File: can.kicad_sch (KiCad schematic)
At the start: 14 parts, among them J1 RJ45_LED_Shielded, J2 RJ45_LED_Shielded, J3 Conn_01x04, SW1 SW_DIP_x02

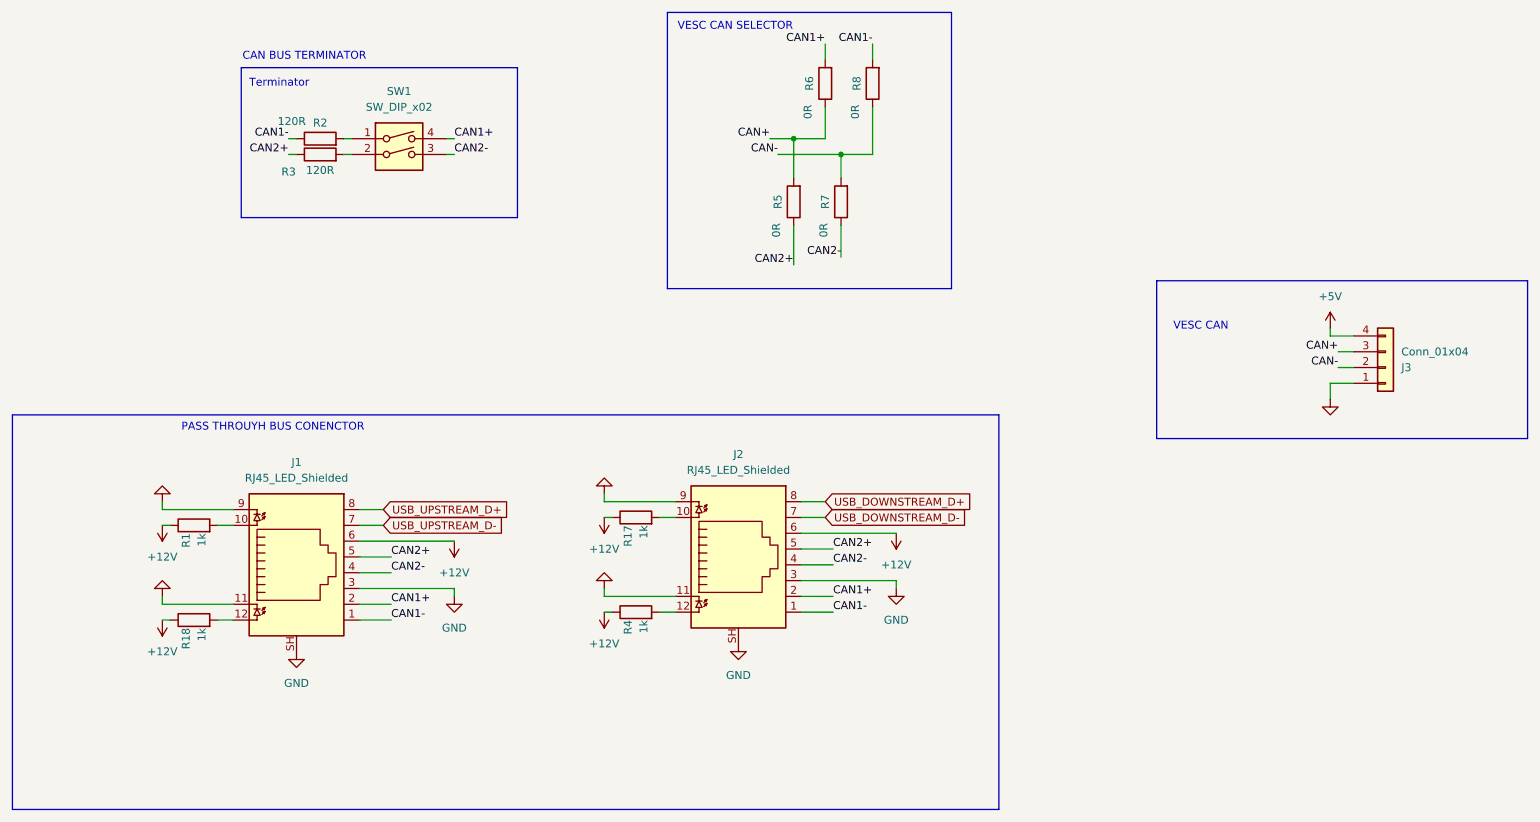
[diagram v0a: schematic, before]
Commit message: rev v3 tiny
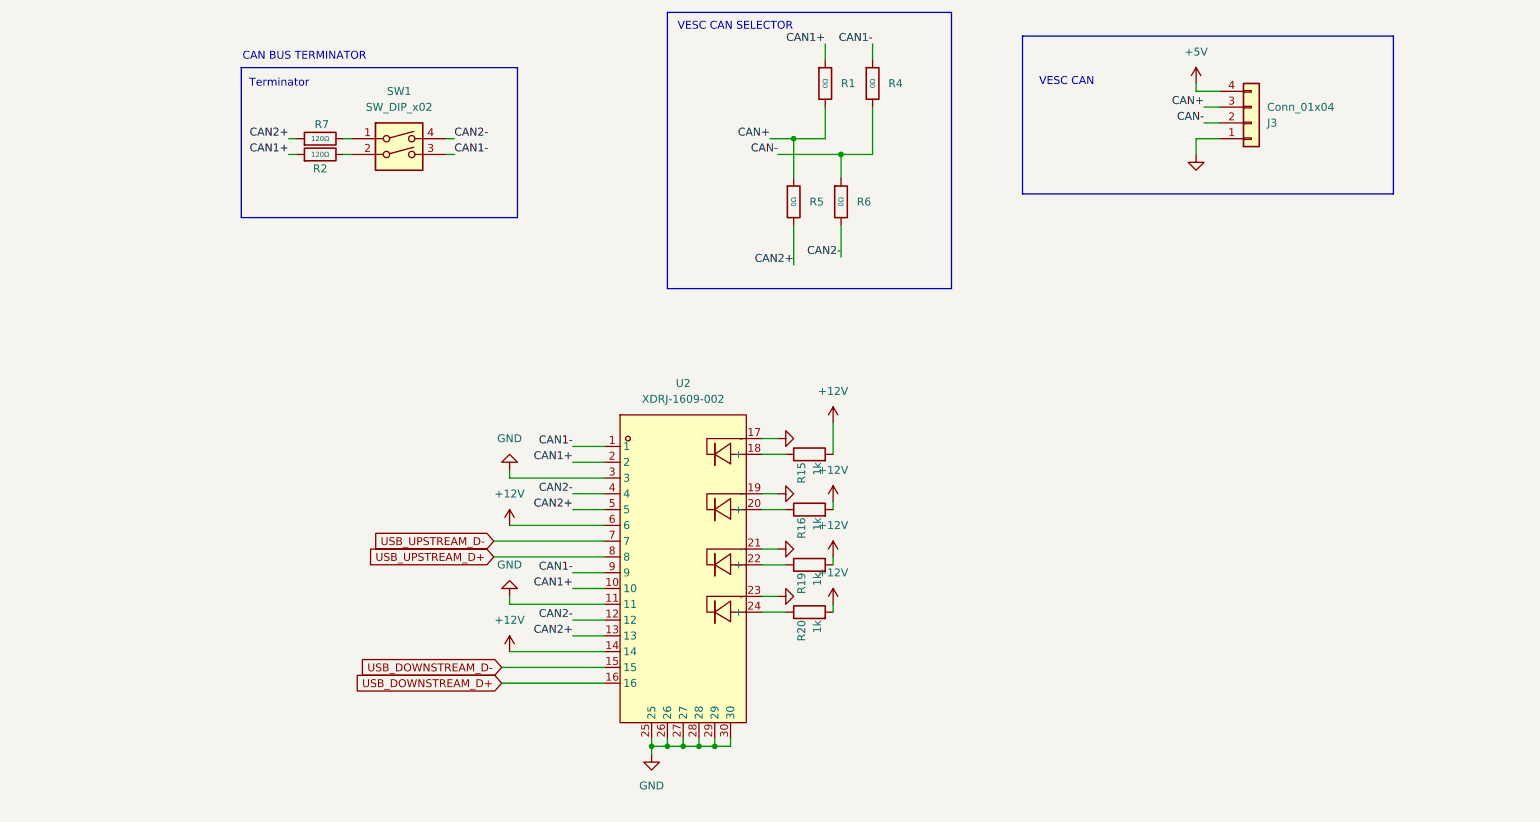
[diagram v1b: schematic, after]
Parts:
- removed J1, J2: RJ45_LED_Shielded, Connector_RJ:RJ45_Amphenol_RJHSE538X, symbol Connector:RJ45_LED_Shielded
- removed R1, R17, R18, R4: 1k, Resistor_SMD:R_0402_1005Metric, symbol Device:R
- removed R2, R3: 120R, Resistor_SMD:R_0603_1608Metric, symbol Device:R
- removed R5, R6, R7, R8: 0R, Resistor_SMD:R_0603_1608Metric, symbol Device:R
- added R1, R4, R5, R6: 0Ω, PCM_JLCPCB:R_0402, symbol PCM_JLCPCB-Resistors:0402,0Ω
- added R15, R16, R19, R20: 1k, Resistor_SMD:R_0402_1005Metric, symbol Device:R
- added R2, R7: 120Ω, PCM_JLCPCB:R_0402, symbol PCM_JLCPCB-Resistors:0402,120Ω
- added U2: XDRJ-1609-002, rj45:RJ45-TH_XDRJ-1609-002, symbol rj45:XDRJ-1609-002
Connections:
- net +12V: now also R15.2, R16.2, R19.2, R20.2, U2.14, U2.6
- net CAN+: now also R1.2, R5.1
- net CAN-: now also R4.2, R6.1
- net CAN1+: now also R1.1, R2.1, U2.10, U2.2; no longer SW1.4
- net CAN1-: now also SW1.3, R4.1, U2.1, U2.9
- net CAN2+: now also R5.2, R7.1, U2.13, U2.5
- net CAN2-: now also SW1.4, R6.2, U2.12, U2.4; no longer SW1.3
- net GND: now also U2.11, U2.17 (-), U2.19 (-), U2.21 (-), U2.23 (-), U2.25, U2.26, U2.27, U2.28, U2.29, U2.3, U2.30
- net USB_DOWNSTREAM_D+: now also U2.16
- net USB_DOWNSTREAM_D-: now also U2.15
- net USB_UPSTREAM_D+: now also U2.8
- net USB_UPSTREAM_D-: now also U2.7
- net at SW1.2: now also R2.2
- net at SW1.1: now also R7.2
- new net: R16.1, U2.20 (+)
- new net: R19.1, U2.22 (+)
- new net: R15.1, U2.18 (+)
- new net: R20.1, U2.24 (+)
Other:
- note removed: "PASS THROUYH BUS CONENCTOR"
- moved on the sheet: J3
